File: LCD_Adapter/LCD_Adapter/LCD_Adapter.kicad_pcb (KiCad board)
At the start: 4 copper layers, 45 x 45 mm, 29 parts, among them J1 Conn_01x10, J2 FH12-30S-0.5SH_55_, J3 Conn_01x22, U1 TLV75801PDBV, U2 TLV75801PDBV, U3 TPS61042DRBR

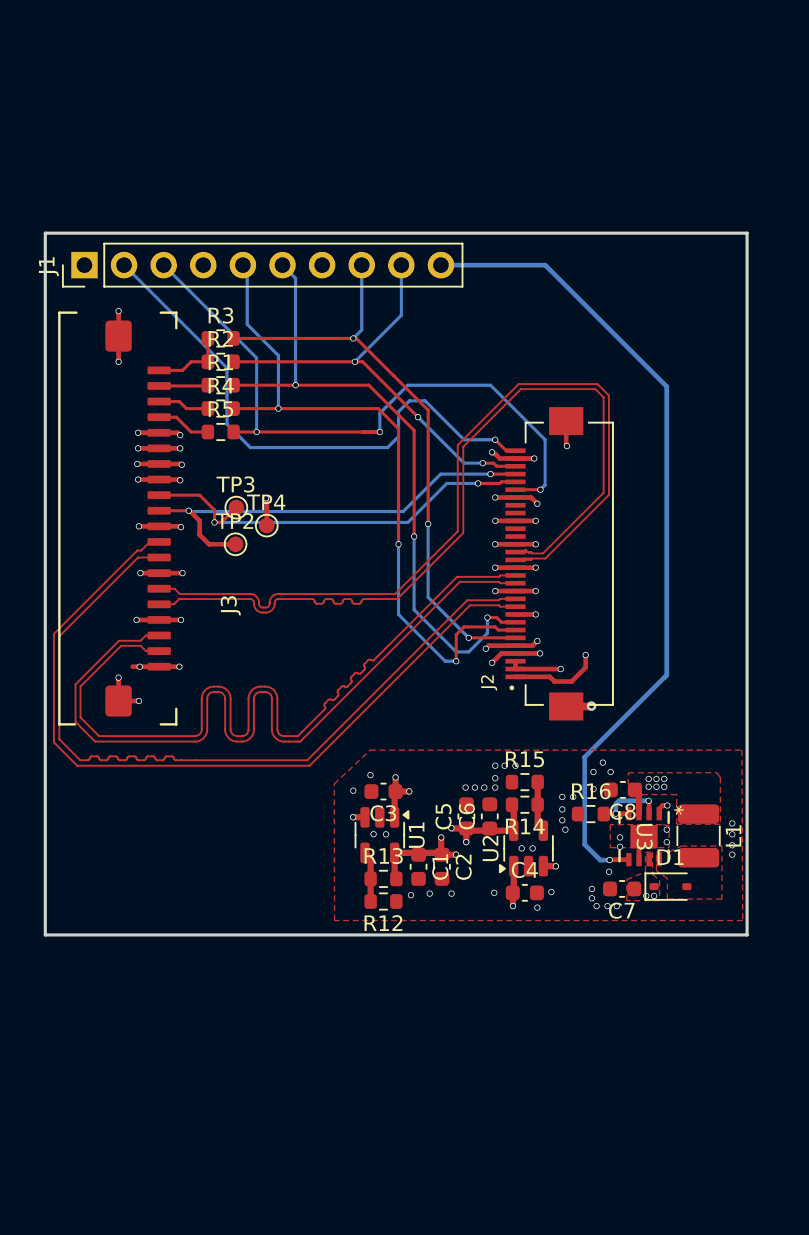
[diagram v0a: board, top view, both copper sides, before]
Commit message: PCD_UPDATE
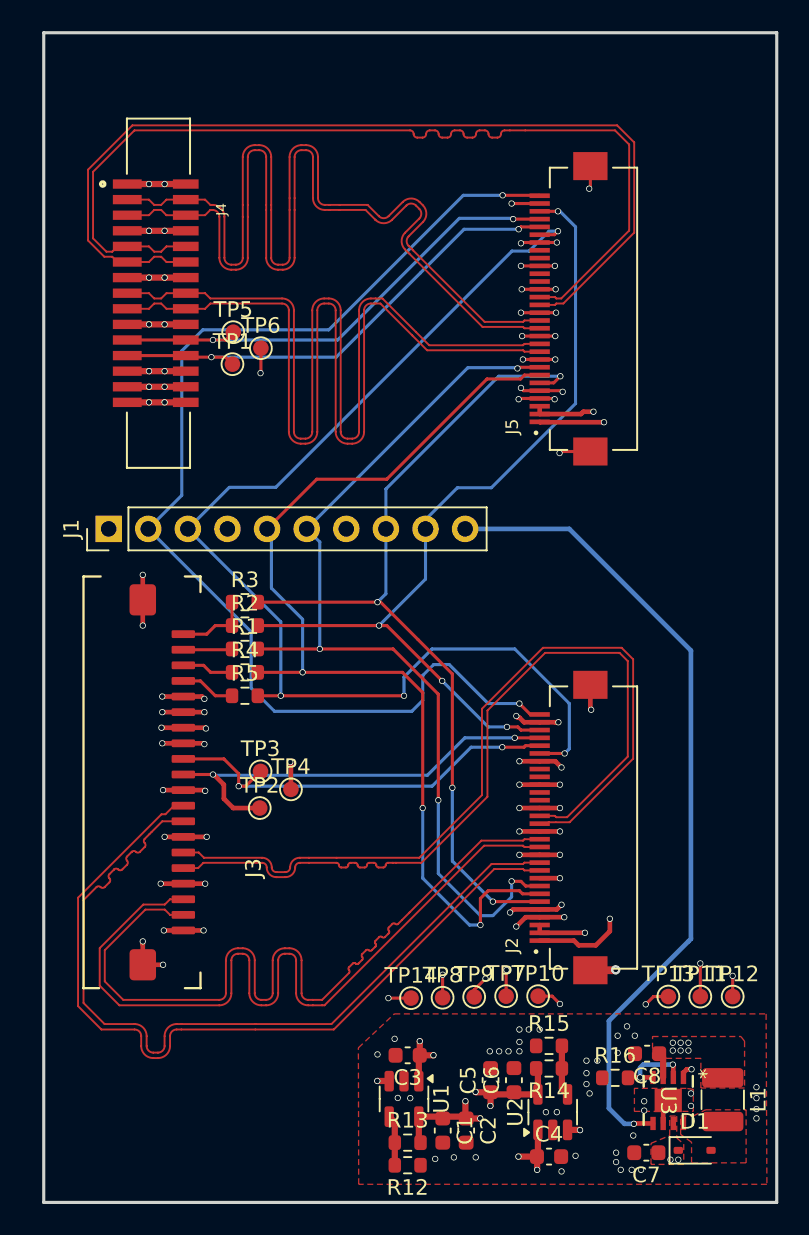
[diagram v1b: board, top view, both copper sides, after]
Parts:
- added J4: 1-1734248-5, lib:TE_1-1734248-5, F.Cu at (103.1, 36.2)
- added J5: FH12-30S-0.5SH_55_, lib:HIROSE_FH12-30S-0.5SH_55_, F.Cu at (127.5, 37.2)
- added TP1: TestPoint, TestPoint:TestPoint_Pad_D1.0mm, F.Cu at (107.8, 40.8)
- added TP10: TestPoint, TestPoint:TestPoint_Pad_D1.0mm, F.Cu at (127.5, 81.3)
- added TP11: TestPoint, TestPoint:TestPoint_Pad_D1.0mm, F.Cu at (137.8, 81.3)
- added TP12: TestPoint, TestPoint:TestPoint_Pad_D1.0mm, F.Cu at (139.9, 81.3)
- added TP13: TestPoint, TestPoint:TestPoint_Pad_D1.0mm, F.Cu at (135.8, 81.3)
- added TP14: TestPoint, TestPoint:TestPoint_Pad_D1.0mm, F.Cu at (119.3, 81.4)
- added TP5: TestPoint, TestPoint:TestPoint_Pad_D1.0mm, F.Cu at (107.9, 38.7)
- added TP6: TestPoint, TestPoint:TestPoint_Pad_D1.0mm, F.Cu at (109.7, 39.7)
- added TP7: TestPoint, TestPoint:TestPoint_Pad_D1.0mm, F.Cu at (125.4, 81.3)
- added TP8: TestPoint, TestPoint:TestPoint_Pad_D1.0mm, F.Cu at (121.3, 81.4)
- added TP9: TestPoint, TestPoint:TestPoint_Pad_D1.0mm, F.Cu at (123.3, 81.3)
- moved C8 17.0 mm to (134.4, 85.0)
- moved J2 17.0 mm to (127.5, 70.5)
- moved R12 17.0 mm to (119.1, 92.1)
- moved R13 17.0 mm to (119.1, 90.7)
- moved R15 17.0 mm to (128.2, 84.5)
- moved TP2 17.0 mm to (109.6, 69.2)
- moved U3 17.0 mm to (135.8, 88.0)
- moved R16 17.0 mm to (132.4, 86.5)
- moved U2 17.0 mm to (128.4, 88.7)
- moved J1 17.0 mm to (99.9, 51.3)
- moved J3 17.0 mm to (109.7, 73.1)
- moved R1 17.0 mm to (108.7, 59.0)
- moved R2 17.0 mm to (108.7, 57.5)
- moved R3 17.0 mm to (108.7, 56.0)
- moved R4 17.0 mm to (108.7, 60.5)
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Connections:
- net / LED_A renamed  LED_A
- net / LED_K renamed  LED_K
- net /CLK_N renamed /STM2LCD/CLK_N
- net /CLK_P renamed /STM2LCD/CLK_P
- net /D0_N renamed /STM2LCD/D0_N
- net /D0_P renamed /STM2LCD/D0_P
- net /D1_N renamed /STM2LCD/D1_N
- net /D1_P renamed /STM2LCD/D1_P
- net /D2_N renamed /STM2LCD/D2_N
- net /D2_P renamed /STM2LCD/D2_P
- net /D3_N renamed /STM2LCD/D3_N
- net /D3_P renamed /STM2LCD/D3_P
- net /DC_LED_PWM renamed DC_LED_PWM
- net /LCM_ID renamed LCM_ID
- net /PWM renamed PWM
- net /RESET renamed RESET
- net /TE renamed TE
- net /TP_INT renamed TP_INT
- net /TP_RES renamed TP_RES
- net /TP_SCL renamed TP_SCL
- net /TP_SDA renamed TP_SDA
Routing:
- net +2V8: track 30.9 -> 98.0 mm, vias 6 -> 10
- net /RPI2LCD/RPI_CLK_P: track 0.00 -> 62.1 mm
- net /RPI2LCD/RPI_CLK_N: track 0.00 -> 61.9 mm
- net /RPI2LCD/RPI_D0_P: track 0.00 -> 61.8 mm
- net /RPI2LCD/RPI_D0_N: track 0.00 -> 61.8 mm
- net /RPI2LCD/RPI_D1_P: track 0.00 -> 61.7 mm
- net /RPI2LCD/RPI_D1_N: track 0.00 -> 61.7 mm
- net +1V8: track 30.6 -> 74.7 mm, vias 4 -> 7
- net  LED_K: track 19.3 -> 61.4 mm, vias 2 -> 4
- net GND: track 44.1 -> 85.9 mm, vias 72 -> 100
- net  LED_A: track 26.9 -> 67.5 mm, vias 3 -> 5
- net LCM_ID: track 35.6 -> 75.0 mm, vias 1 -> 2
- net TP_INT: track 42.6 -> 74.4 mm, vias 3 -> 4
- net RPI_TP_SDA: track 0.00 -> 31.5 mm, vias 0 -> 2
- net RPI_TP_SCL: track 0.00 -> 31.2 mm, vias 0 -> 2
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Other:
- board size 45 x 45 mm -> 47 x 75 mm
